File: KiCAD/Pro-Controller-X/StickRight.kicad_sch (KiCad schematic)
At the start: 2 parts, among them J1 Conn_01x05_Pin

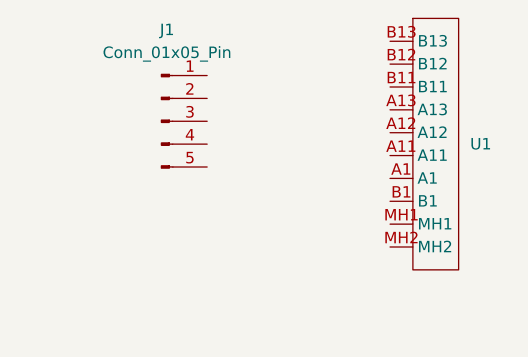
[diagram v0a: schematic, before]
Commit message: Joystick Boards done
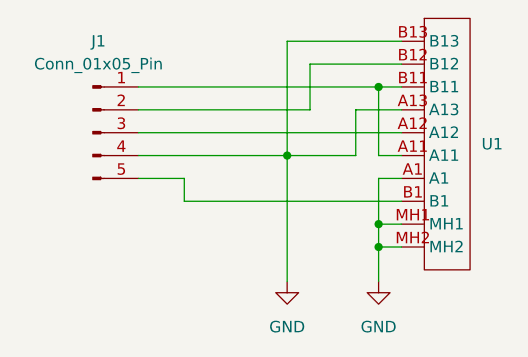
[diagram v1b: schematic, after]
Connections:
- net GND: now reaches U1.A1
- net GND: now also J1.4 (Pin_4), U1.A13, U1.B13, U1.MH1, U1.MH2
- net at U1.A11: now also J1.1 (Pin_1), U1.B11
- net at U1.A12: now also J1.3 (Pin_3)
- net at U1.B1: now also J1.5 (Pin_5)
- net at U1.B12: now also J1.2 (Pin_2)
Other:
- moved on the sheet: U1
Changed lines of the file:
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@@
 (kicad_sch (version 20230121) (generator eeschema)
   (paper "A2")
-  (symbol (lib_id "ProControllerX:StickBox") (at 262.89 190.5 0) (unit 1)
+  (junction (at 259.08 195.58) (diameter 0) (color 0 0 0 0)
+  )
+  (junction (at 248.92 203.2) (diameter 0) (color 0 0 0 0)
+  )
+  (junction (at 259.08 213.36) (diameter 0) (color 0 0 0 0)
+  )
+  (junction (at 259.08 210.82) (diameter 0) (color 0 0 0 0)
+  )
+  (wire (pts (xy 232.41 198.12) (xy 251.46 198.12))
+    (stroke (width 0) (type default))
+  )
+  (wire (pts (xy 232.41 205.74) (xy 237.49 205.74))
+    (stroke (width 0) (type default))
+  )
+  (wire (pts (xy 261.62 198.12) (xy 256.54 198.12))
+    (stroke (width 0) (type default))
+  )
+  (wire (pts (xy 259.08 210.82) (xy 259.08 213.36))
+    (stroke (width 0) (type default))
+  )
+  (wire (pts (xy 259.08 217.17) (xy 259.08 213.36))
+    (stroke (width 0) (type default))
+  )
+  (wire (pts (xy 259.08 195.58) (xy 261.62 195.58))
+    (stroke (width 0) (type default))
+  )
+  (wire (pts (xy 261.62 208.28) (xy 237.49 208.28))
+    (stroke (width 0) (type default))
+  )
+  (wire (pts (xy 251.46 193.04) (xy 251.46 198.12))
+    (stroke (width 0) (type default))
+  )
+  (wire (pts (xy 232.41 200.66) (xy 261.62 200.66))
+    (stroke (width 0) (type default))
+  )
+  (wire (pts (xy 248.92 203.2) (xy 248.92 217.17))
+    (stroke (width 0) (type default))
+  )
+  (wire (pts (xy 248.92 190.5) (xy 261.62 190.5))
+    (stroke (width 0) (type default))
+  )
+  (wire (pts (xy 259.08 213.36) (xy 261.62 213.36))
+    (stroke (width 0) (type default))
+  )
+  (wire (pts (xy 261.62 203.2) (xy 259.08 203.2))
+    (stroke (width 0) (type default))
+  )
+  (wire (pts (xy 261.62 193.04) (xy 251.46 193.04))
+    (stroke (width 0) (type default))
+  )
+  (wire (pts (xy 232.41 203.2) (xy 248.92 203.2))
+    (stroke (width 0) (type default))
+  )
+  (wire (pts (xy 261.62 205.74) (xy 259.08 205.74))
+    (stroke (width 0) (type default))
+  )
+  (wire (pts (xy 259.08 203.2) (xy 259.08 195.58))
+    (stroke (width 0) (type default))
+  )
+  (wire (pts (xy 256.54 203.2) (xy 248.92 203.2))
+    (stroke (width 0) (type default))
+  )
+  (wire (pts (xy 232.41 195.58) (xy 259.08 195.58))
+    (stroke (width 0) (type default))
+  )
+  (wire (pts (xy 259.08 205.74) (xy 259.08 210.82))
+    (stroke (width 0) (type default))
+  )
+  (wire (pts (xy 261.62 210.82) (xy 259.08 210.82))
+    (stroke (width 0) (type default))
+  )
+  (wire (pts (xy 256.54 198.12) (xy 256.54 203.2))
+    (stroke (width 0) (type default))
+  )
+  (wire (pts (xy 237.49 208.28) (xy 237.49 205.74))
+    (stroke (width 0) (type default))
+  )
+  (wire (pts (xy 248.92 203.2) (xy 248.92 190.5))
+    (stroke (width 0) (type default))
+  )
+  (symbol (lib_id "ProControllerX:StickBox") (at 264.16 190.5 0) (unit 1)
     (in_bom yes) (on_board yes) (dnp no) (fields_autoplaced)
-    (property "Reference" "U1" (at 269.24 201.93 0)
+    (property "Reference" "U1" (at 270.51 201.93 0)
       (effects (font (size 1.27 1.27)) (justify left))
     )
-    (property "Value" "~" (at 260.35 190.5 0)
+    (property "Value" "~" (at 261.62 190.5 0)
       (effects (font (size 1.27 1.27)))
     )
-    (property "Footprint" "ProControllerX:RJoystick" (at 260.35 190.5 0)
+    (property "Footprint" "ProControllerX:RJoystick" (at 261.62 190.5 0)
       (effects (font (size 1.27 1.27)) hide)
     )
-    (property "Datasheet" "" (at 260.35 190.5 0)
+    (property "Datasheet" "" (at 261.62 190.5 0)
       (effects (font (size 1.27 1.27)) hide)
     )
@@
     )
   )
-  (symbol (lib_id "Connector:Conn_01x05_Pin") (at 234.95 199.39 0) (unit 1)
+  (symbol (lib_id "power:GND") (at 248.92 217.17 0) (unit 1)
     (in_bom yes) (on_board yes) (dnp no) (fields_autoplaced)
-    (property "Reference" "J1" (at 235.585 189.23 0)
+    (property "Reference" "#PWR02" (at 248.92 223.52 0)
+      (effects (font (size 1.27 1.27)) hide)
+    )
+    (property "Value" "GND" (at 248.92 222.25 0)
       (effects (font (size 1.27 1.27)))
     )
-    (property "Value" "Conn_01x05_Pin" (at 235.585 191.77 0)
+    (property "Footprint" "" (at 248.92 217.17 0)
+      (effects (font (size 1.27 1.27)) hide)
+    )
+    (property "Datasheet" "" (at 248.92 217.17 0)
+      (effects (font (size 1.27 1.27)) hide)
+    )
+    (pin "1")
+    (instances
+      (project "StickRight"
+        (path "/40a7657d-c4d7-4ebc-b606-0c6932d6f433"
+          (reference "#PWR02") (unit 1)
+        )
+      )
+    )
+  )
+  (symbol (lib_id "power:GND") (at 259.08 217.17 0) (unit 1)
+    (in_bom yes) (on_board yes) (dnp no) (fields_autoplaced)
+    (property "Reference" "#PWR01" (at 259.08 223.52 0)
+      (effects (font (size 1.27 1.27)) hide)
+    )
+    (property "Value" "GND" (at 259.08 222.25 0)
       (effects (font (size 1.27 1.27)))
     )
-    (property "Footprint" "Connector_PinHeader_2.54mm:PinHeader_1x05_P2.54mm_Horizontal" (at 234.95 199.39 0)
+    (property "Footprint" "" (at 259.08 217.17 0)
       (effects (font (size 1.27 1.27)) hide)
     )
-    (property "Datasheet" "~" (at 234.95 199.39 0)
+    (property "Datasheet" "" (at 259.08 217.17 0)
       (effects (font (size 1.27 1.27)) hide)
     )
+    (pin "1")
+    (instances
+      (project "StickRight"
+        (path "/40a7657d-c4d7-4ebc-b606-0c6932d6f433"
+          (reference "#PWR01") (unit 1)
+        )
+      )
+    )
+  )
+  (symbol (lib_id "Connector:Conn_01x05_Pin") (at 227.33 200.66 0) (unit 1)
+    (in_bom yes) (on_board yes) (dnp no) (fields_autoplaced)
+    (property "Reference" "J1" (at 227.965 190.5 0)
+      (effects (font (size 1.27 1.27)))
+    )
+    (property "Value" "Conn_01x05_Pin" (at 227.965 193.04 0)
+      (effects (font (size 1.27 1.27)))
+    )
+    (property "Footprint" "Connector_PinHeader_2.54mm:PinHeader_1x05_P2.54mm_Horizontal" (at 227.33 200.66 0)
+      (effects (font (size 1.27 1.27)) hide)
+    )
+    (property "Datasheet" "~" (at 227.33 200.66 0)
+      (effects (font (size 1.27 1.27)) hide)
+    )
